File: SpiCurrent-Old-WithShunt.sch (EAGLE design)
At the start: 58 parts, among them IC1 AD822N, IC2 AD822N, IC3 ACS758LCB-050B-PFF-T, IC4 ACS758LCB-050B-PFF-T, U1 HIP4081AIPZ

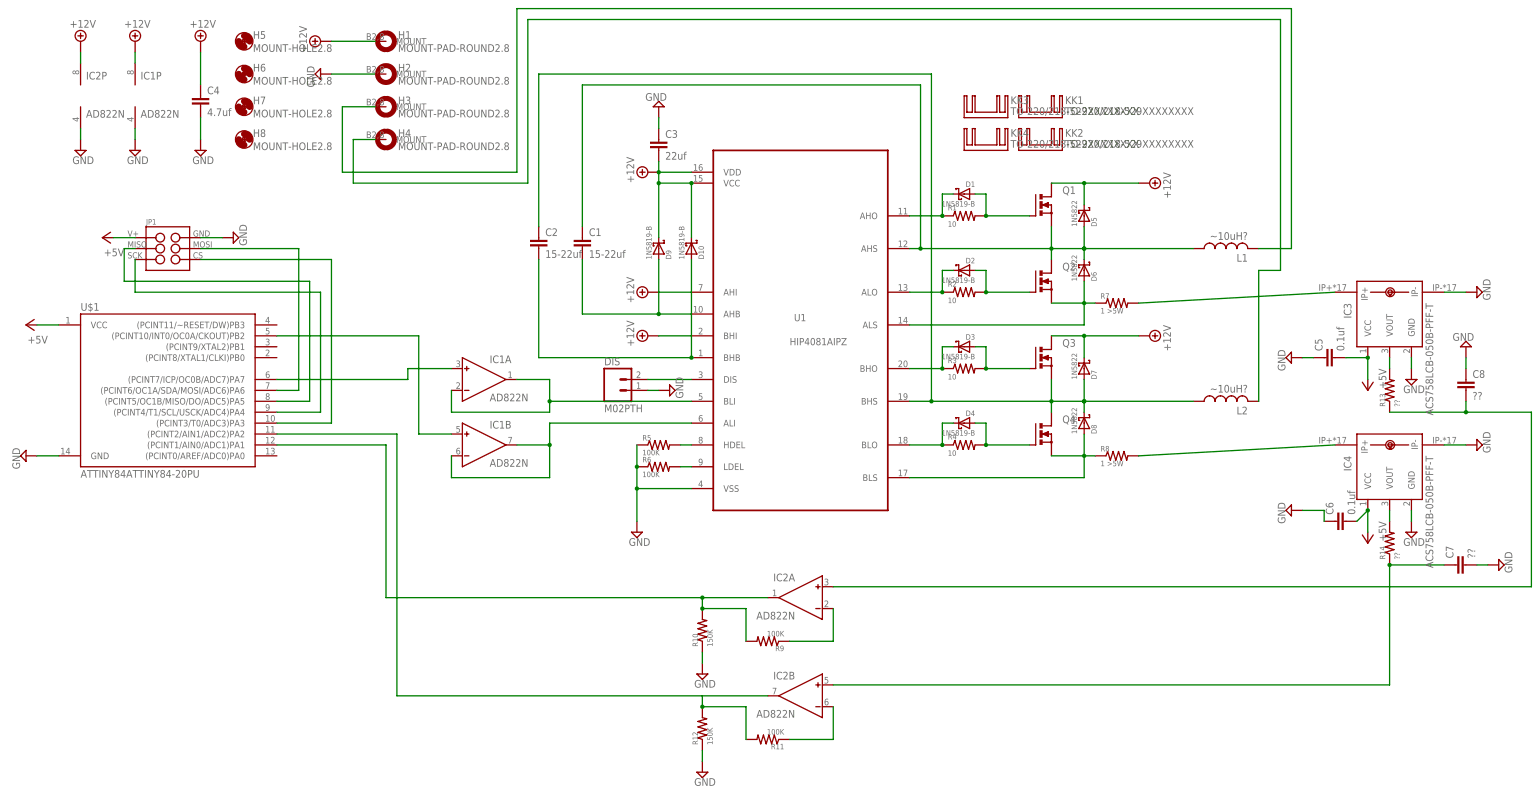
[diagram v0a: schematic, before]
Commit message: barely begun layout
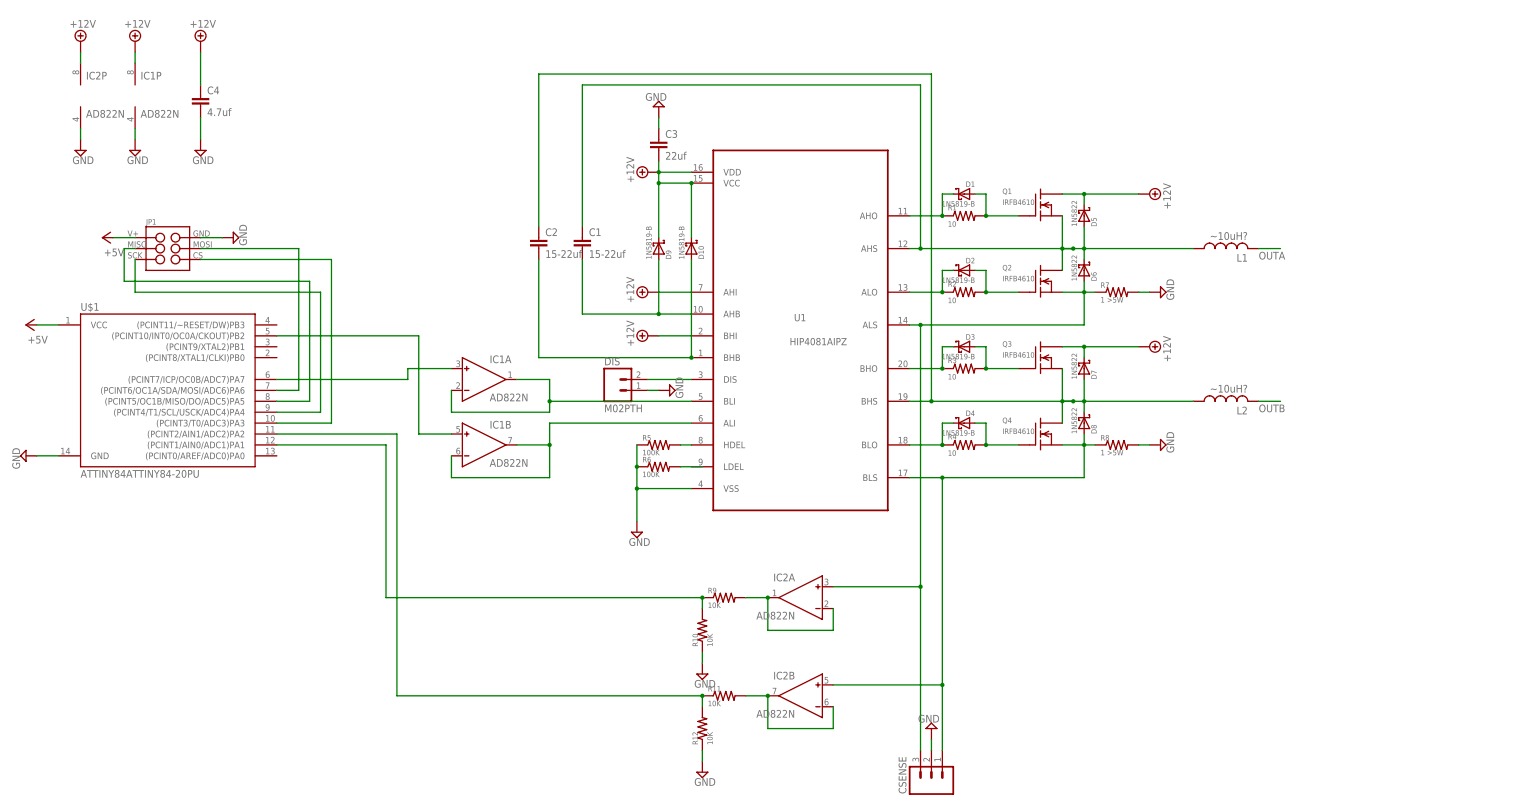
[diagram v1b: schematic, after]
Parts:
- removed C5, C6: 0.1uf, rcl:C-EU050-055X075
- removed C7, C8: ??, rcl:C-EU050-055X075
- removed H1, H2, H3, H4: MOUNT-PAD-ROUND2.8, holes-custom:MOUNT-PAD-ROUND2.8
- removed H5, H6, H7, H8: MOUNT-HOLE2.8, holes:MOUNT-HOLE2.8
- removed IC3, IC4: ACS758LCB-050B-PFF-T, allegro:ACS758LCB-050B-PFF-T
- removed KK1, KK2, KK3, KK4: TO-220/218-529XXXXXXXX, heatsink-aavid:TO-220/218-529XXXXXXXX
- removed R13, R14: ??, resistor-custom:R-US_0207/10
- added CSENSE: (no value), SparkFun-Connectors:M03PTH
- Q1, Q2, Q3, Q4: value (none) -> IRFB4610; device transistor-power:PMOSFET_NTO220BV -> CustomParts:IRFB4610
- R10, R12: value 150K -> 10K
- R11, R9: value 100K -> 10K
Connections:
- removed net N$27: IC4.IP+, R8.2
- removed net N$31: IC3.IP+, R7.2
- removed net N$32: C8.2, IC2A.IN+, R13.1
- removed net N$33: C7.1, IC2B.IN+, R14.1
- removed net N$34: IC3.VOUT, R13.2
- removed net N$35: IC4.VOUT, R14.2
- removed net N$36: H3.MOUNT, L1.2
- removed net N$37: H4.MOUNT, L2.2
- new net OUTA: L1.2
- new net OUTB: L2.2
- net +12V: no longer H1.MOUNT
- net +5V: no longer C5.2, C6.2, IC3.VCC, IC4.VCC
- net GND: now also CSENSE.2, R7.2, R8.2; no longer C5.1, C6.1, C7.2, C8.1, H2.MOUNT, IC3.GND, IC3.IP-, IC4.GND, IC4.IP-
- net N$13: no longer U1.LDEL
- net N$15: now also CSENSE.3, IC2A.IN+
- net N$16: now also CSENSE.1, IC2B.IN+
- net N$26: now also R10.2, U$1.(PCINT1/AIN0/ADC1)PA1; no longer IC2A.IN-
- net N$28: now also IC2A.IN-; no longer R10.2, U$1.(PCINT1/AIN0/ADC1)PA1
- net N$29: now also IC2B.IN-; no longer R12.2, U$1.(PCINT2/AIN1/ADC2)PA2
- net N$30: now also R12.2, U$1.(PCINT2/AIN1/ADC2)PA2; no longer IC2B.IN-
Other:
- moved on the sheet: R11, R7, R8, R9
